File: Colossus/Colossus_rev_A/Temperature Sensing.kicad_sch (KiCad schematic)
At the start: 4 parts

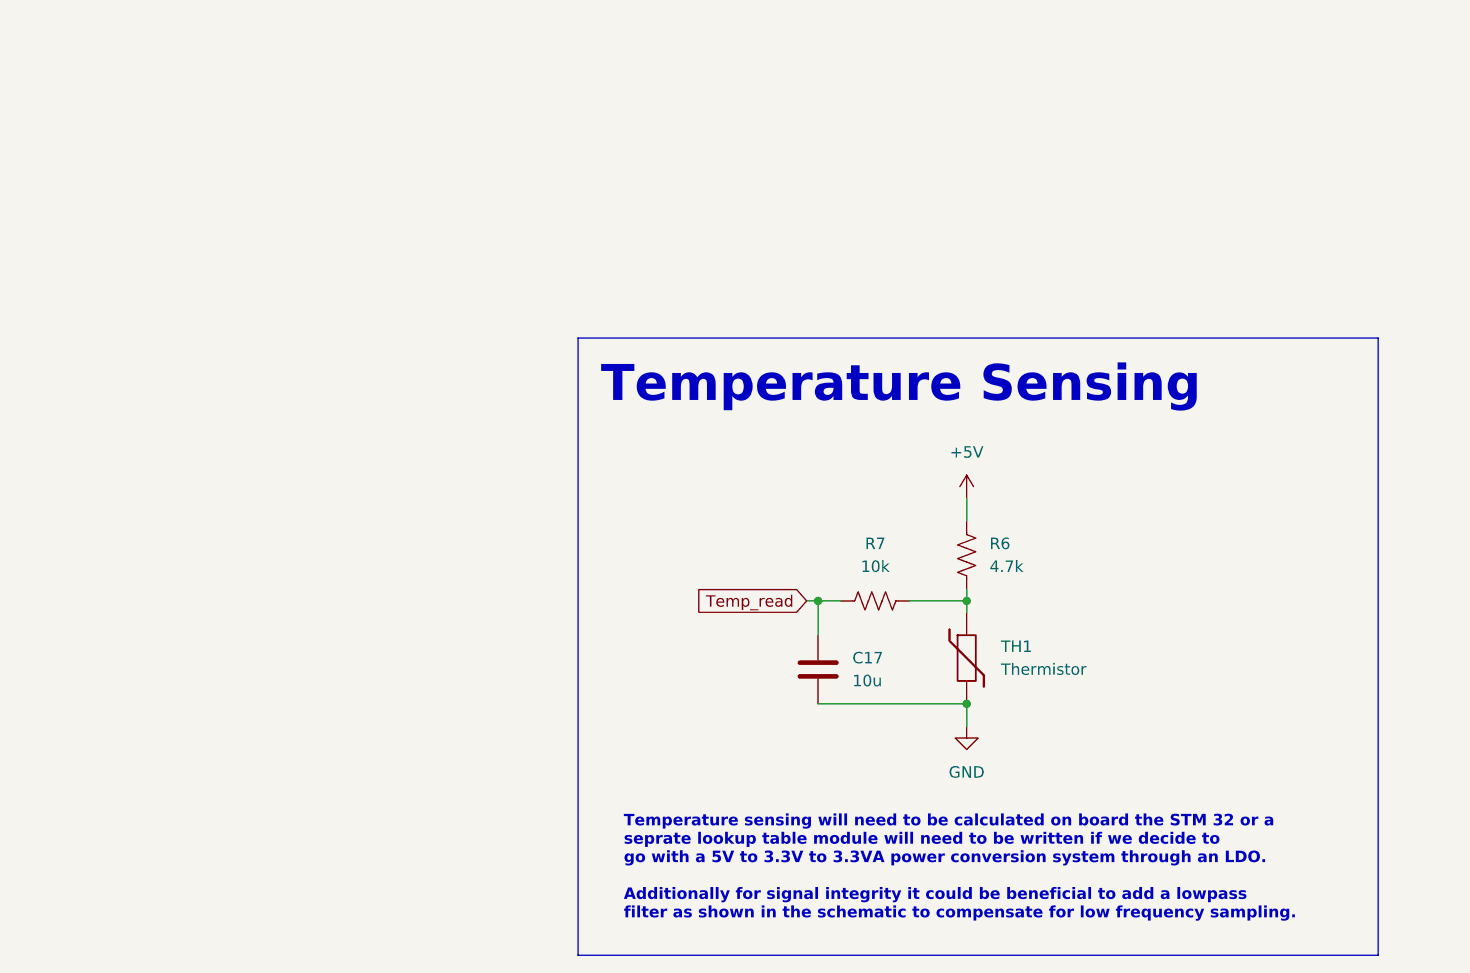
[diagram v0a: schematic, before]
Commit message: pushing to save
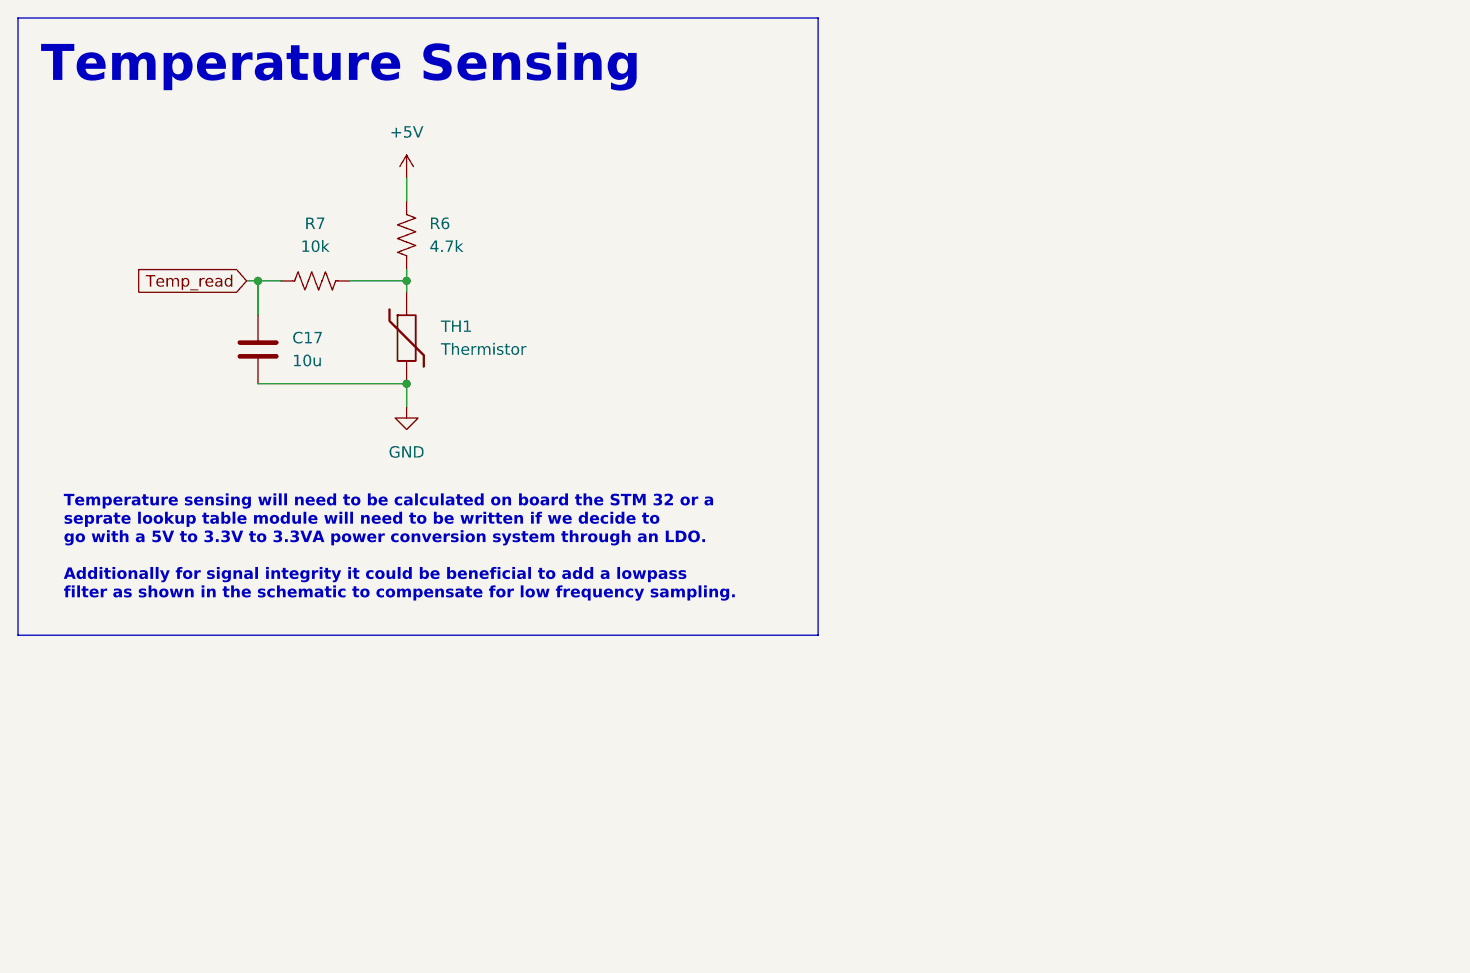
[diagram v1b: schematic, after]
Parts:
- C17: footprint (none) -> Capacitor_SMD:C_0201_0603Metric
- R6, R7, TH1: footprint (none) -> Resistor_SMD:R_01005_0402Metric
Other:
- moved on the sheet: C17, R6, R7, TH1
